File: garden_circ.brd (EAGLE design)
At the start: 87.8 x 59 mm, 47 parts, among them IC1 MEGA8-P, IC2 74HC595D, IC3 74HC595D, IC4 7805DT, J1 POWER_JACKSLT, Q3 MOSFET-NCHANNELBSS123LT1G

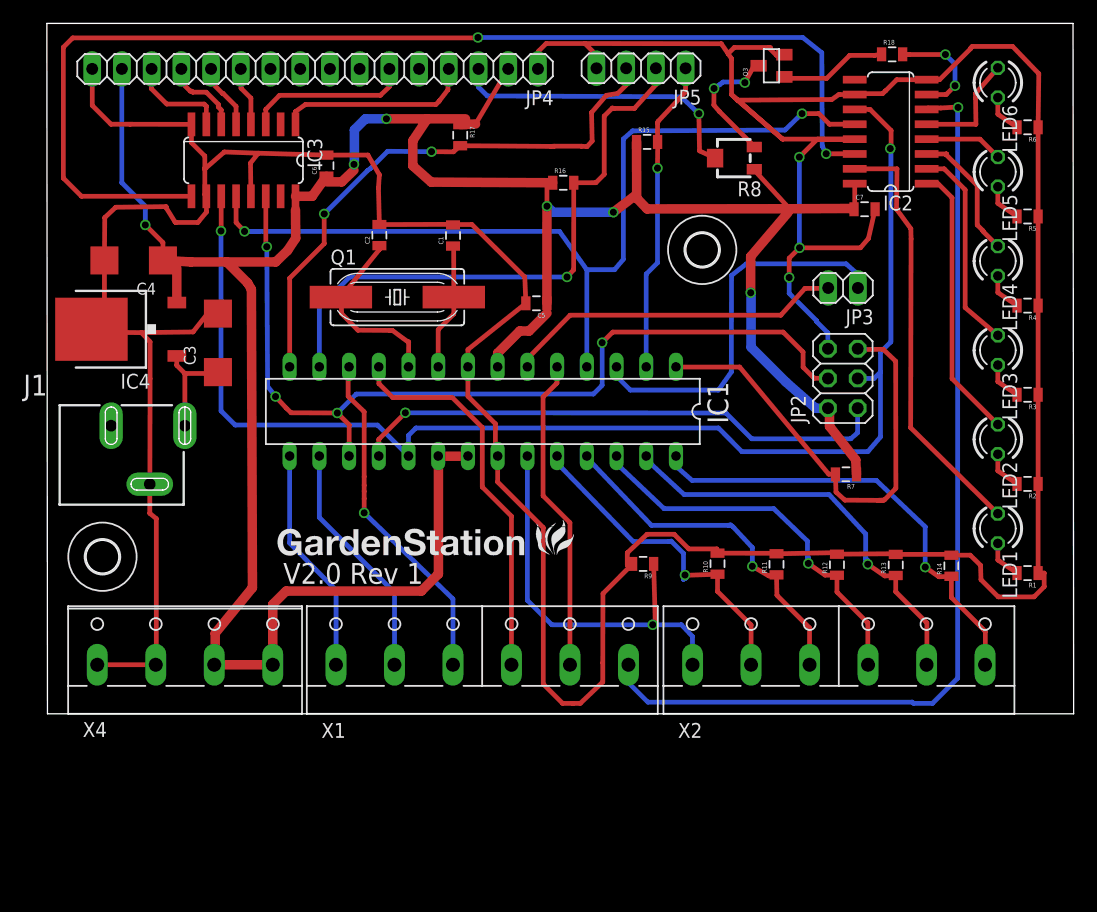
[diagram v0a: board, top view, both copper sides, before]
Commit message: Added a few tweaks and power light
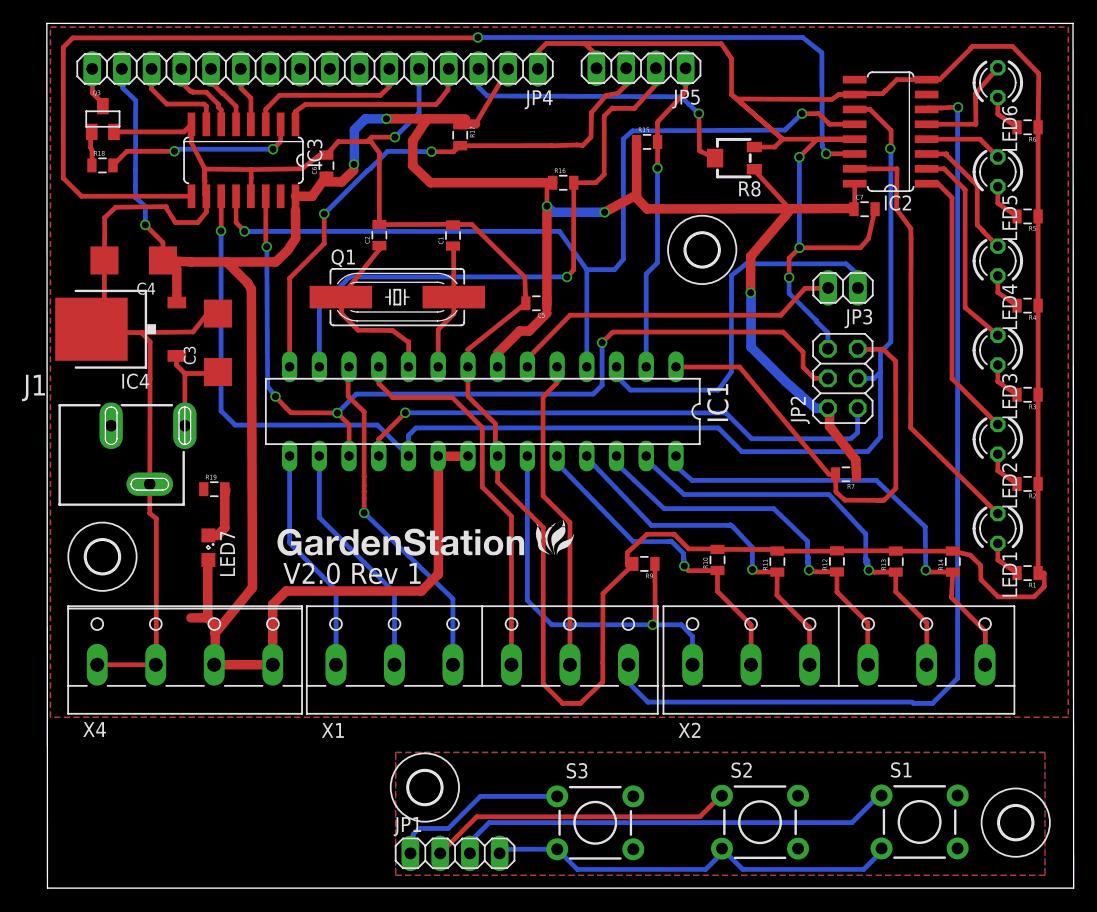
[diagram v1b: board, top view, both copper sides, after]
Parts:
- added H3, H4: MOUNT-HOLE2.8, holes:2,8
- added JP1: (no value), pinhead:1X04
- added LED7: (no value), led:SML0805
- added R19: 220, SparkFun-Resistors:0805
- added S1, S2, S3: SWITCH-MOMENTARY-2PTH, SparkFun-Electromechanical:TACTILE-PTH
- moved R18 68.2 mm to (0.94, 71.7)
- moved Q3 57.3 mm to (0.98, 75.6), turned to 0 degrees
- moved R14 0.38 mm to (73.6, 37.8)
- moved R10 0.32 mm to (53.5, 38.0)
- moved R12 0.28 mm to (63.7, 37.8)
- moved R13 0.28 mm to (68.7, 37.8)
- moved R11 0.24 mm to (58.6, 37.8)
- moved R9 0.11 mm to (47.3, 37.6)
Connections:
- new net N$69: IC3.2, R18.2
- new net N$70: JP1.2, S2.1
- new net N$71: JP1.3, S1.1
- new net N$72: JP1.4, S1.3, S2.3, S3.3
- new net N$73: LED7.C, R19.2
- net GND: now also JP4.5, R19.1, R8.3; no longer JP4.16
- net N$66: now also JP1.1, S3.1; no longer Q3.3, R8.3
- net N$67: now also JP4.16, Q3.3; no longer IC2.7, R18.2
- net VCC: now also LED7.A
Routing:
- net N$71: track 0.00 -> 37.8 mm
- net N$72: track 0.00 -> 36.1 mm
- net N$70: track 0.00 -> 26.1 mm
- net N$69: track 0.00 -> 16.7 mm, vias 0 -> 2
- net VCC: track 243.9 -> 251.9 mm
- net N$68: track 9.77 -> 3.00 mm
- net N$67: track 9.39 -> 3.56 mm, vias 2 -> 0
- net N$73: track 0.00 -> 5.12 mm
- net GND: track 376.9 -> 381.8 mm, vias 3 -> 4
- net N$66: track 11.3 -> 15.4 mm, vias 2 -> 0
- net N$33: track 33.7 -> 34.8 mm
- net N$34: track 36.4 -> 37.3 mm
- added copper zone on layer 1, net GND
- added copper zone on layer 16, net GND
- added copper zone on layer 1, net N$72
- added copper zone on layer 16, net N$72
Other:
- board size 87.8 x 59 mm -> 87.8 x 73.9 mm
